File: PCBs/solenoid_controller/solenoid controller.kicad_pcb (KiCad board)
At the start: 2 copper layers, 87.9 x 65 mm, 66 parts, among them J1 Conn_02x03_Odd_Even, J2 Conn_02x03_Odd_Even, J3 Conn_02x04_Odd_Even, J4 SWD, J5 Solenoid, J6 GND_CONN, J7 28V_CONN, Q1 Q_NMOS_SDG, U1 23LCV512, U2 AMS1117-3.3, U3 AOZ1284, U4 AMS1117-5.0, U5 STM32F030K6Tx, U6 MIC4416, U7 ACS712xLCTR-30A, Y1 12Mhz

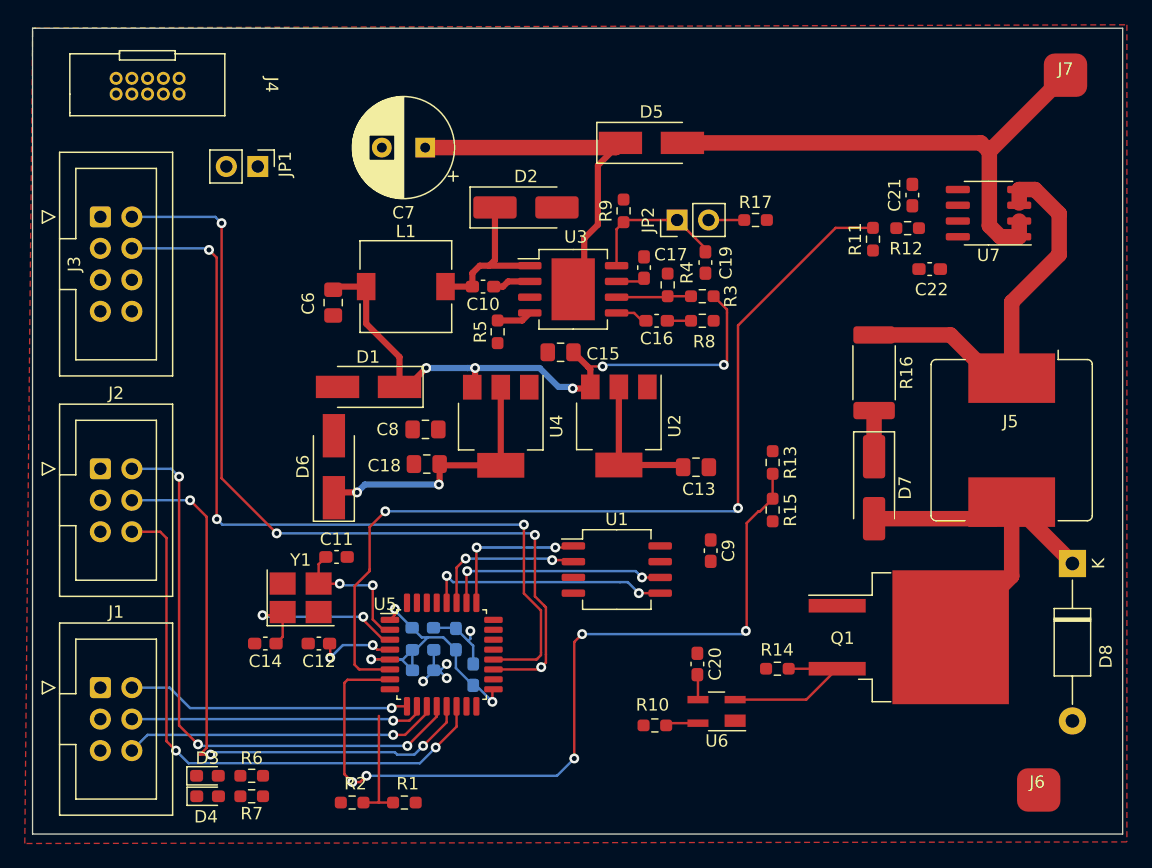
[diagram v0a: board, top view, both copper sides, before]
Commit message: solenoid controller finished
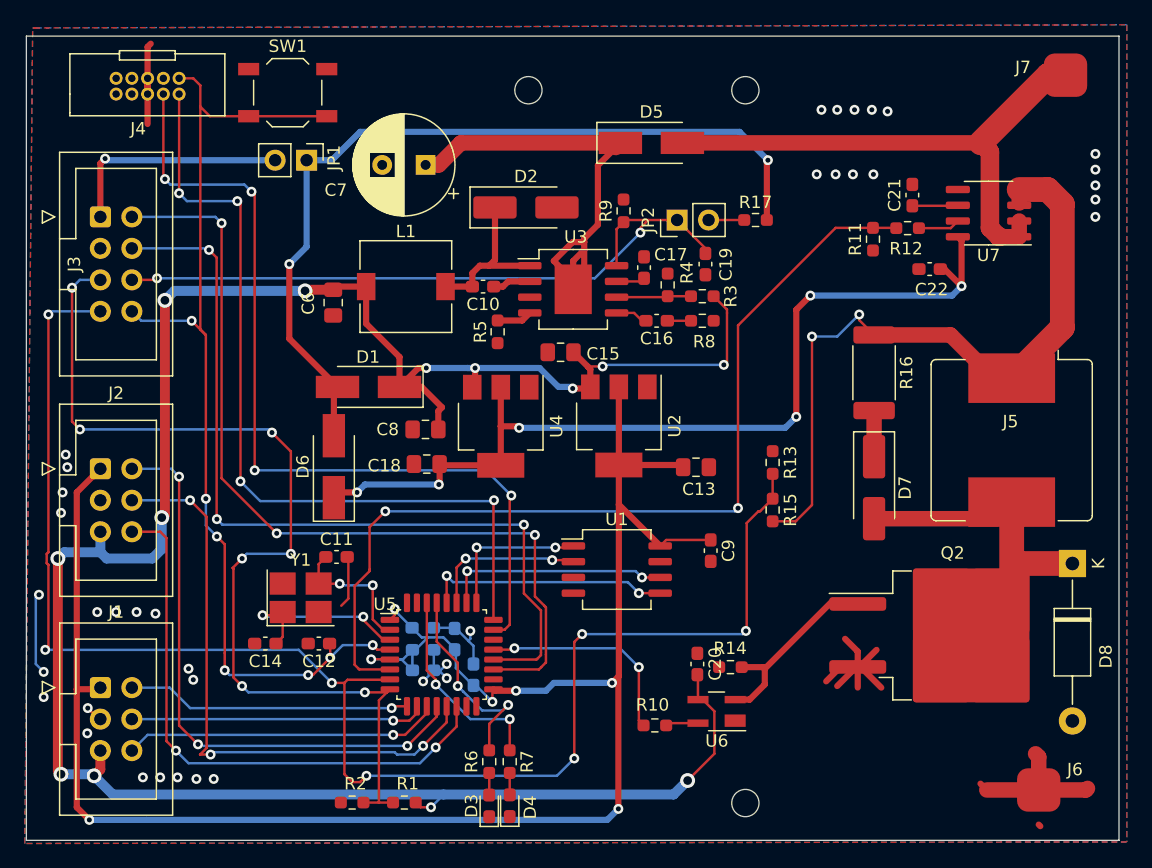
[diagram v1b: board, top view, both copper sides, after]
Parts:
- removed Q1: Q_NMOS_SDG, Package_TO_SOT_SMD:TO-263-2
- added Q2: Q_NMOS_GDS, Package_TO_SOT_SMD:TO-263-2, F.Cu at (154.2, 119.0)
- added REF**: MountingHole_2.2mm_M2, MountingHole:MountingHole_2.2mm_M2, F.Cu at (137.5, 75.0)
- added REF**: MountingHole_2.2mm_M2, MountingHole:MountingHole_2.2mm_M2, F.Cu at (137.5, 132.5)
- added REF**: MountingHole_2.2mm_M2, MountingHole:MountingHole_2.2mm_M2, F.Cu at (120.0, 75.0)
- added SW1: SW_Push, Button_Switch_SMD:SW_SPST_TL3342, F.Cu at (100.6, 75.2)
- moved D4 24.4 mm to (118.5, 132.7), turned to 90 degrees
- moved D3 22.9 mm to (116.8, 132.7), turned to 90 degrees
- moved R7 21.0 mm to (118.5, 129.2), turned to 90 degrees
- moved R6 19.2 mm to (116.8, 129.2), turned to 90 degrees
- moved JP1 3.97 mm to (102.1, 80.6)
- moved R14 3.79 mm to (136.3, 121.5)
- moved C7 1.40 mm to (111.7, 81.0)
- moved C19 0.13 mm to (134.3, 89.0)
- moved C1 0.10 mm to (114.0, 119.3)
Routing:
- net +12V: track 53.5 -> 186.9 mm, vias 5 -> 13
- net +3V3: track 36.7 -> 158.6 mm, vias 3 -> 7
- net /NRST: track 6.55 -> 83.0 mm, vias 2 -> 7
- net /SWDIO: track 0.00 -> 70.4 mm, vias 0 -> 4
- net /BUCK_VOL_DIV: track 9.38 -> 79.4 mm, vias 0 -> 7
- net +5VP: track 0.00 -> 68.5 mm, vias 0 -> 2
- net /SWCLK: track 0.00 -> 66.5 mm, vias 0 -> 4
- net /MOSFET_VOL_DIV: track 68.0 -> 124.8 mm, vias 5 -> 7
- net +5V: track 21.9 -> 75.3 mm, vias 2 -> 6
- net GND: track 11.6 -> 60.9 mm, vias 4 -> 38
- net /BUCK_ENABLE: track 11.6 -> 55.5 mm, vias 0 -> 2
- net Net-(J5-Pin_1): track 32.5 -> 57.3 mm, vias 0 -> 2
- net Net-(J3-Pin_1): track 0.00 -> 19.0 mm, vias 0 -> 1
- net /MOSFET_CTRL: track 0.00 -> 17.3 mm, vias 0 -> 2
- net Net-(U5-PB6): track 0.00 -> 16.8 mm, vias 0 -> 2
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- added copper zone on B.Cu, net GND
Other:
- board size 87.9 x 65 mm -> 88.1 x 64.9 mm
